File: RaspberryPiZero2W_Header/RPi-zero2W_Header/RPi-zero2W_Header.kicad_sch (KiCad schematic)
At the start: 2 parts

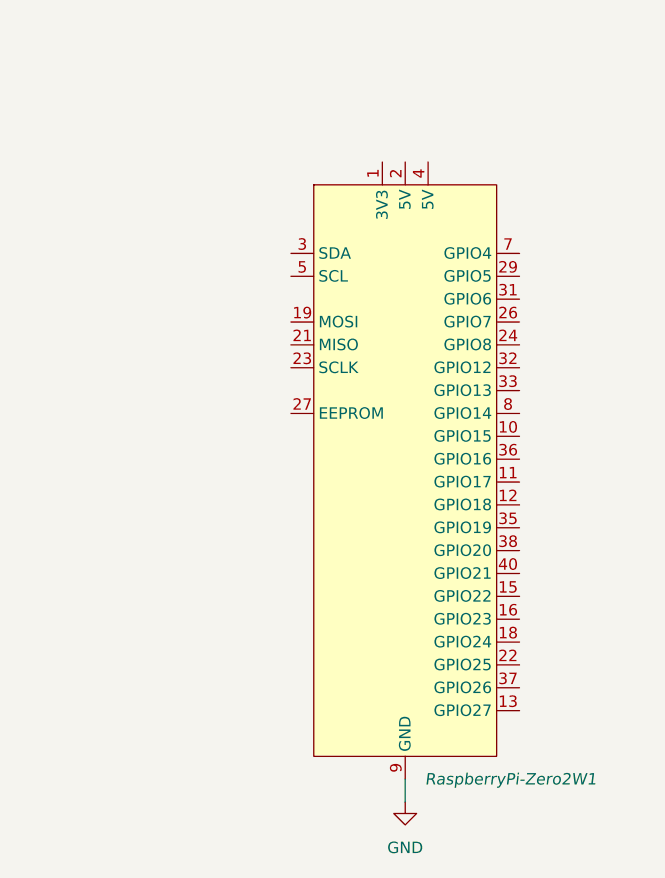
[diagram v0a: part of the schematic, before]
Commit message: .
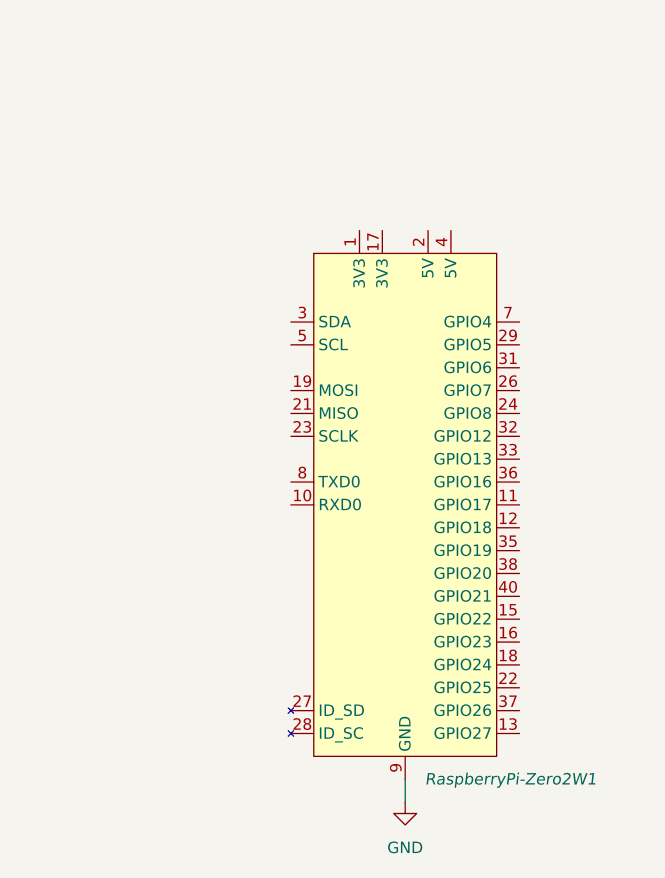
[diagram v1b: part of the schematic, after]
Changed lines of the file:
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@@
-	)
-	(symbol
-		(lib_id "Alexander KiCad Libraries:BRD_RPI-Zero-2W")
-		(at 170.18 50.8 0)
-		(unit 1)
-		(exclude_from_sim no)
-		(in_bom yes)
-		(on_board yes)
-		(dnp no)
-		(fields_autoplaced yes)
-		(property "Reference" "RaspberryPi-Zero2W1"
-			(at 177.4541 119.38 0)
-			(effects
-				(font
-					(size 1.27 1.27)
-					(italic yes)
-				)
-				(justify left)
-			)
-		)
-		(property "Value" "~"
-			(at 177.4541 120.65 0)
-			(effects
-				(font
-					(size 1.27 1.27)
-				)
-				(justify left)
-			)
-		)
-		(property "Footprint" "Alexander Footprint Library:RaspberryPiZero2W"
-			(at 170.942 35.052 0)
-			(effects
-				(font
-					(size 1.27 1.27)
-				)
-				(hide yes)
-			)
-		)
-		(property "Datasheet" ""
-			(at 175.26 50.8 0)
-			(effects
-				(font
-					(size 1.27 1.27)
-				)
-				(hide yes)
-			)
-		)
-		(property "Description" "Raspberry Pi Zero 2 W"
-			(at 175.514 83.312 90)
-			(effects
-				(font
-					(size 1.27 1.27)
-				)
-				(hide yes)
-			)
-		)
-		(pin "34"
-		)
-		(pin "9"
-		)
-		(pin "16"
-		)
-		(pin "18"
-		)
-		(pin "13"
-		)
-		(pin "29"
-		)
-		(pin "14"
-		)
-		(pin "10"
-		)
-		(pin "30"
-		)
-		(pin "37"
-		)
-		(pin "36"
-		)
-		(pin "12"
-		)
-		(pin "7"
-		)
-		(pin "15"
-		)
-		(pin "8"
-		)
-		(pin "25"
-		)
-		(pin "40"
-		)
-		(pin "24"
-		)
-		(pin "23"
-		)
-		(pin "27"
-		)
-		(pin "39"
-		)
-		(pin "32"
-		)
-		(pin "35"
-		)
-		(pin "22"
-		)
-		(pin "38"
-		)
-		(pin "33"
-		)
-		(pin "5"
-		)
-		(pin "11"
-		)
-		(pin "26"
-		)
-		(pin "20"
-		)
-		(pin "21"
-		)
-		(pin "31"
-		)
-		(pin "4"
-		)
-		(pin "3"
-		)
-		(pin "2"
-		)
-		(pin "1"
-		)
-		(pin "19"
-		)
-		(instances
-			(project ""
-				(path "/bc57b58b-4c14-4a77-83b7-825e5df65c1a"
-					(reference "RaspberryPi-Zero2W1")
-					(unit 1)
-				)
-			)
-		)
 	)
 	(symbol
@@
 					(unit 1)
 				)
+			)
+		)
+	)
+	(symbol
+		(lib_id "Alexander KiCad Libraries:BRD_RPI-Zero-2W")
+		(at 170.18 58.42 0)
+		(unit 1)
+		(exclude_from_sim no)
+		(in_bom yes)
+		(on_board yes)
+		(dnp no)
+		(fields_autoplaced yes)
+		(property "Reference" "RaspberryPi-Zero2W1"
+			(at 177.4541 119.38 0)
+			(effects
+				(font
+					(size 1.27 1.27)
+					(italic yes)
+				)
+				(justify left)
+			)
+		)
+		(property "Value" "~"
+			(at 177.4541 120.65 0)
+			(effects
+				(font
+					(size 1.27 1.27)
+				)
+				(justify left)
+			)
+		)
+		(property "Footprint" "Alexander Footprint Library:RaspberryPiZero2W"
+			(at 170.942 42.672 0)
+			(effects
+				(font
+					(size 1.27 1.27)
+				)
+				(hide yes)
+			)
+		)
+		(property "Datasheet" ""
+			(at 175.26 58.42 0)
+			(effects
+				(font
+					(size 1.27 1.27)
+				)
+				(hide yes)
+			)
+		)
+		(property "Description" "Raspberry Pi Zero 2 W"
+			(at 175.514 90.932 90)
+			(effects
+				(font
+					(size 1.27 1.27)
+				)
+				(hide yes)
+			)
+		)
+		(pin "25"
+		)
+		(pin "29"
+		)
+		(pin "31"
+		)
+		(pin "36"
+		)
+		(pin "17"
+		)
+		(pin "30"
+		)
+		(pin "38"
+		)
+		(pin "11"
+		)
+		(pin "13"
+		)
+		(pin "20"
+		)
+		(pin "22"
+		)
+		(pin "15"
+		)
+		(pin "23"
+		)
+		(pin "27"
+		)
+		(pin "32"
+		)
+		(pin "35"
+		)
+		(pin "39"
+		)
+		(pin "8"
+		)
+		(pin "9"
+		)
+		(pin "10"
+		)
+		(pin "18"
+		)
+		(pin "33"
+		)
+		(pin "1"
+		)
+		(pin "12"
+		)
+		(pin "14"
+		)
+		(pin "2"
+		)
+		(pin "3"
+		)
+		(pin "37"
+		)
+		(pin "4"
+		)
+		(pin "40"
+		)
+		(pin "5"
+		)
+		(pin "34"
+		)
+		(pin "26"
+		)
+		(pin "7"
+		)
+		(pin "16"
+		)
+		(pin "24"
+		)
+		(pin "19"
+		)
+		(pin "28"
+		)
+		(pin "21"
+		)
+		(instances
+			(project ""
+				(path "/bc57b58b-4c14-4a77-83b7-825e5df65c1a"
+					(reference "RaspberryPi-Zero2W1")
+					(unit 1)
+				)
